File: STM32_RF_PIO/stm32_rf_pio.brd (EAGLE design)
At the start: 80 x 39.4 mm, 10 parts, among them IC1 ULN2804A, IC2 ULN2804A, IC3 ULN2804A, X1 22-23-2081, X2 22-23-2081, X3 22-23-2081, X4 Outputs Power

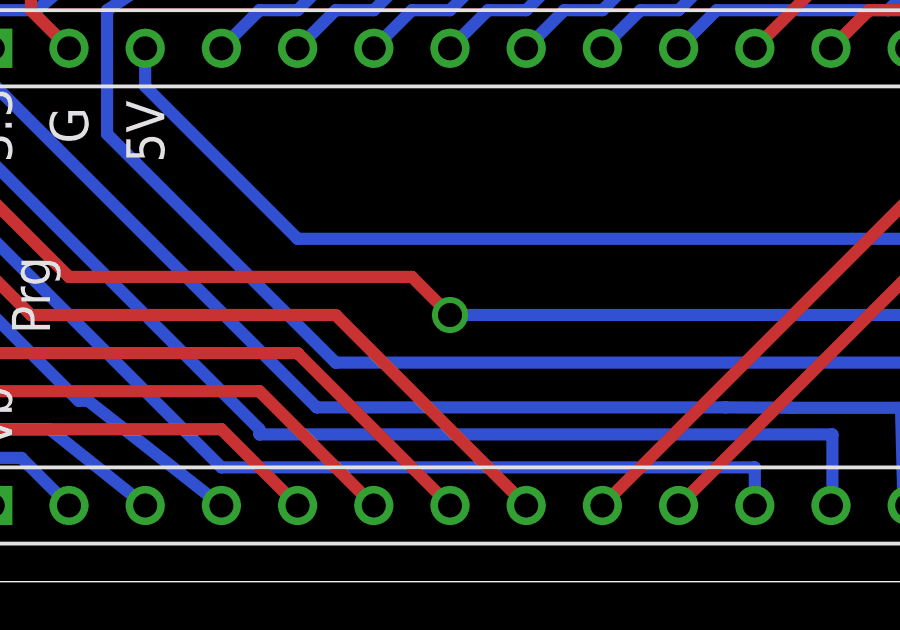
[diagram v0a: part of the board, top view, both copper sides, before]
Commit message: preparing production 1
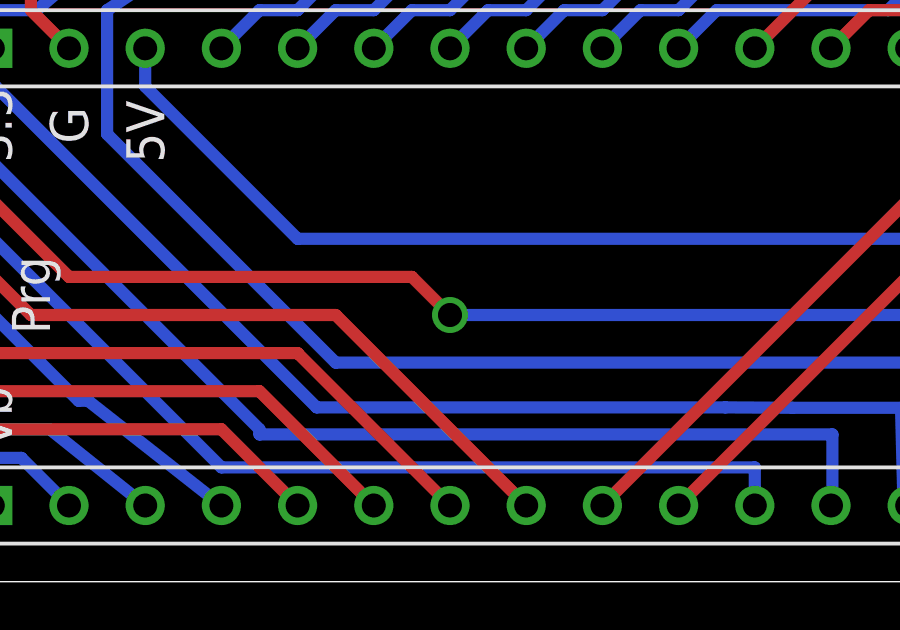
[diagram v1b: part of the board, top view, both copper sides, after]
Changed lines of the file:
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@@
 <layers>
 <layer number="1" name="Top" color="4" fill="1" visible="yes" active="yes"/>
-<layer number="16" name="Bottom" color="1" fill="1" visible="no" active="yes"/>
+<layer number="16" name="Bottom" color="1" fill="1" visible="yes" active="yes"/>
 <layer number="17" name="Pads" color="2" fill="1" visible="yes" active="yes"/>
 <layer number="18" name="Vias" color="2" fill="1" visible="yes" active="yes"/>
@@
 <layer number="20" name="Dimension" color="15" fill="1" visible="yes" active="yes"/>
 <layer number="21" name="tPlace" color="7" fill="1" visible="yes" active="yes"/>
-<layer number="22" name="bPlace" color="7" fill="1" visible="no" active="yes"/>
+<layer number="22" name="bPlace" color="7" fill="1" visible="yes" active="yes"/>
 <layer number="23" name="tOrigins" color="15" fill="1" visible="yes" active="yes"/>
-<layer number="24" name="bOrigins" color="15" fill="1" visible="no" active="yes"/>
+<layer number="24" name="bOrigins" color="15" fill="1" visible="yes" active="yes"/>
 <layer number="25" name="tNames" color="7" fill="1" visible="yes" active="yes"/>
-<layer number="26" name="bNames" color="7" fill="1" visible="no" active="yes"/>
+<layer number="26" name="bNames" color="7" fill="1" visible="yes" active="yes"/>
 <layer number="27" name="tValues" color="7" fill="1" visible="yes" active="yes"/>
-<layer number="28" name="bValues" color="7" fill="1" visible="no" active="yes"/>
+<layer number="28" name="bValues" color="7" fill="1" visible="yes" active="yes"/>
 <layer number="29" name="tStop" color="7" fill="3" visible="no" active="yes"/>
 <layer number="30" name="bStop" color="7" fill="6" visible="no" active="yes"/>
@@
 </class>
 </classes>
-<designrules name="default">
+<designrules name="EagleRules">
 <description language="de">&lt;b&gt;EAGLE Design Rules&lt;/b&gt;
 &lt;p&gt;
@@
 necessary adjustments and save your customized
 design rules under a new name.</description>
+<description language="zh">&lt;b&gt;NOA-Labs EAGLE Design Rules&lt;/b&gt;
+</description>
 <param name="layerSetup" value="(1*16)"/>
 <param name="mtCopper" value="0.035mm 0.035mm 0.035mm 0.035mm 0.035mm 0.035mm 0.035mm 0.035mm 0.035mm 0.035mm 0.035mm 0.035mm 0.035mm 0.035mm 0.035mm 0.035mm"/>
 <param name="mtIsolate" value="1.5mm 0.15mm 0.2mm 0.15mm 0.2mm 0.15mm 0.2mm 0.15mm 0.2mm 0.15mm 0.2mm 0.15mm 0.2mm 0.15mm 0.2mm"/>
-<param name="mdWireWire" value="8mil"/>
-<param name="mdWirePad" value="8mil"/>
-<param name="mdWireVia" value="8mil"/>
-<param name="mdPadPad" value="8mil"/>
-<param name="mdPadVia" value="8mil"/>
-<param name="mdViaVia" value="8mil"/>
-<param name="mdSmdPad" value="8mil"/>
-<param name="mdSmdVia" value="8mil"/>
-<param name="mdSmdSmd" value="8mil"/>
+<param name="mdWireWire" value="7mil"/>
+<param name="mdWirePad" value="7mil"/>
+<param name="mdWireVia" value="7mil"/>
+<param name="mdPadPad" value="7mil"/>
+<param name="mdPadVia" value="7mil"/>
+<param name="mdViaVia" value="7mil"/>
+<param name="mdSmdPad" value="0mil"/>
+<param name="mdSmdVia" value="0mil"/>
+<param name="mdSmdSmd" value="0mil"/>
 <param name="mdViaViaSameLayer" value="8mil"/>
 <param name="mnLayersViaInSmd" value="2"/>
-<param name="mdCopperDimension" value="40mil"/>
-<param name="mdDrill" value="8mil"/>
+<param name="mdCopperDimension" value="20mil"/>
+<param name="mdDrill" value="10mil"/>
 <param name="mdSmdStop" value="0mil"/>
-<param name="msWidth" value="10mil"/>
-<param name="msDrill" value="24mil"/>
-<param name="msMicroVia" value="9.99mm"/>
+<param name="msWidth" value="7mil"/>
+<param name="msDrill" value="12mil"/>
+<param name="msMicroVia" value="12mil"/>
 <param name="msBlindViaRatio" value="0.5"/>
 <param name="rvPadTop" value="0.25"/>
@@
 <param name="rlMinPadBottom" value="10mil"/>
 <param name="rlMaxPadBottom" value="20mil"/>
-<param name="rlMinViaOuter" value="8mil"/>
+<param name="rlMinViaOuter" value="6mil"/>
 <param name="rlMaxViaOuter" value="20mil"/>
-<param name="rlMinViaInner" value="8mil"/>
+<param name="rlMinViaInner" value="6mil"/>
 <param name="rlMaxViaInner" value="20mil"/>
 <param name="rlMinMicroViaOuter" value="4mil"/>
@@
 <param name="psTop" value="-1"/>
 <param name="psBottom" value="-1"/>
-<param name="psFirst" value="-1"/>
+<param name="psFirst" value="0"/>
 <param name="psElongationLong" value="100"/>
 <param name="psElongationOffset" value="100"/>
 <param name="mvStopFrame" value="1"/>
 <param name="mvCreamFrame" value="0"/>
-<param name="mlMinStopFrame" value="4mil"/>
-<param name="mlMaxStopFrame" value="4mil"/>
+<param name="mlMinStopFrame" value="2mil"/>
+<param name="mlMaxStopFrame" value="2mil"/>
 <param name="mlMinCreamFrame" value="0mil"/>
 <param name="mlMaxCreamFrame" value="0mil"/>
-<param name="mlViaStopLimit" value="0mil"/>
+<param name="mlViaStopLimit" value="25mil"/>
 <param name="srRoundness" value="0"/>
 <param name="srMinRoundness" value="0mil"/>
@@
 <param name="checkAngle" value="0"/>
 <param name="checkFont" value="1"/>
-<param name="checkRestrict" value="1"/>
+<param name="checkRestrict" value="0"/>
 <param name="useDiameter" value="13"/>
 <param name="maxErrors" value="50"/>
